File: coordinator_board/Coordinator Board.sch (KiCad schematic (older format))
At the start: 9 parts, among them P1 LCD, P2 Serial

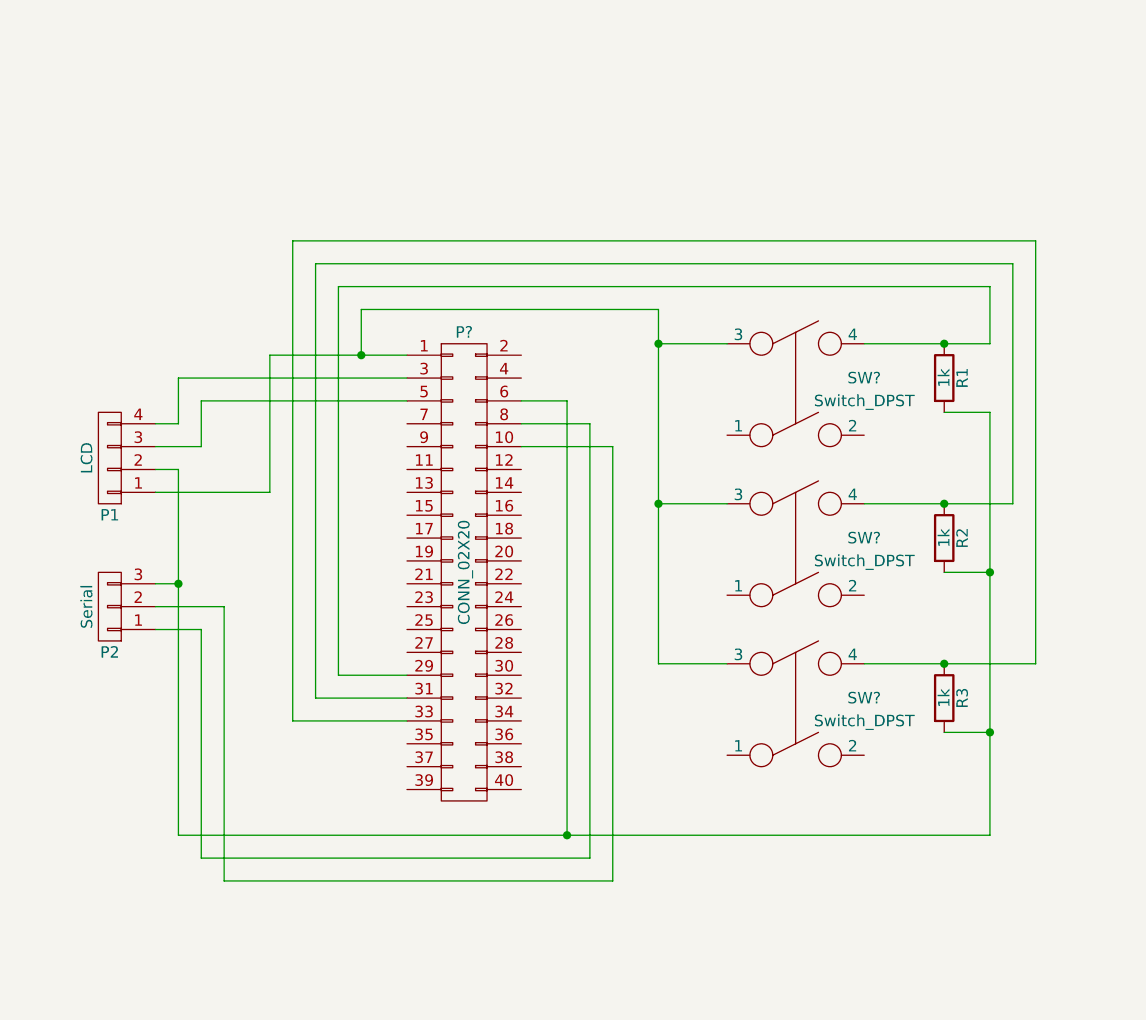
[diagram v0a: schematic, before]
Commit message: Finished v1 of the board
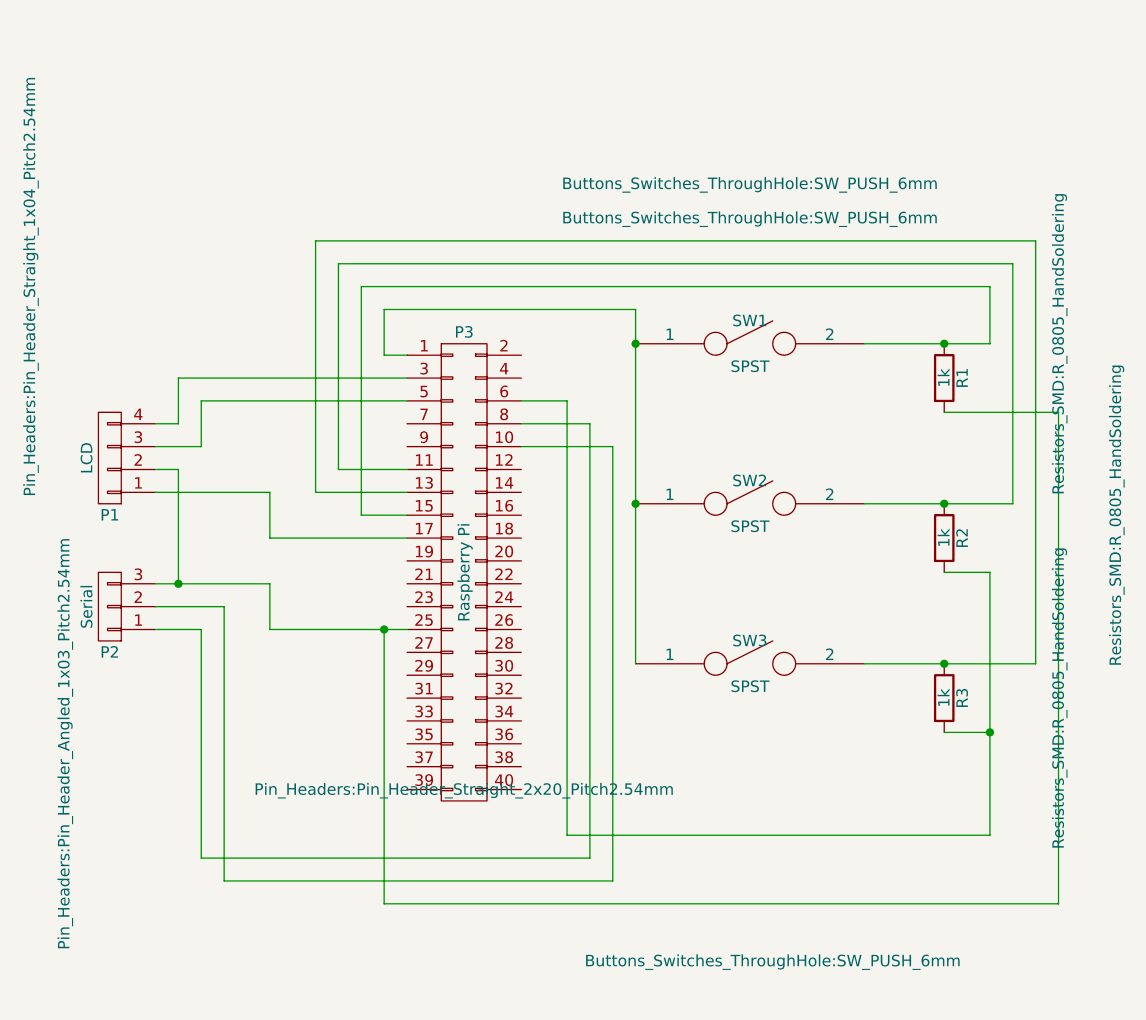
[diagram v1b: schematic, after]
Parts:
- removed SW? (x3): Switch_DPST, symbol Switch_DPST
- added SW1, SW2, SW3: SPST, Buttons_Switches_ThroughHole:SW_PUSH_6mm, symbol SPST
- P1: footprint (none) -> Pin_Headers:Pin_Header_Straight_1x04_Pitch2.54mm
- P2: footprint (none) -> Pin_Headers:Pin_Header_Angled_1x03_Pitch2.54mm
- P3: renamed from P?; value CONN_02X20 -> Raspberry Pi; footprint (none) -> Pin_Headers:Pin_Header_Straight_2x20_Pitch2.54mm
- R1, R2, R3: footprint (none) -> Resistors_SMD:R_0805_HandSoldering
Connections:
- net at P3.1 (P1): now also SW1.1, SW2.1, SW3.1; no longer P1.1 (P1)
- net at P3.11 (P11): now also R2.1, SW2.2
- net at P3.13 (P13): now also R3.1, SW3.2
- net at P3.15 (P15): now also R1.1, SW1.2
- net at P3.17 (P17): now also P1.1 (P1)
- net at P3.25 (P25): now also P1.2 (P2), P2.3 (P3), R1.2
- net at P3.29 (P29): no longer R1.1
- net at P3.31 (P31): no longer R2.1
- net at P3.33 (P33): no longer R3.1
- net at P3.6 (P6), R2.2, R3.2: no longer P1.2 (P2), P2.3 (P3), R1.2
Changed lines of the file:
@@
 $EndDescr
 $Comp
-L CONN_02X20 P?
+L CONN_02X20 P3
 U 1 1 586759B9
 P 3950 3850
-F 0 "P?" H 3950 4900 50  0000 C CNN
-F 1 "CONN_02X20" V 3950 3850 50  0000 C CNN
-F 2 "" H 3950 2900 50  0000 C CNN
+F 0 "P3" H 3950 4900 50  0000 C CNN
+F 1 "Raspberry Pi" V 3950 3850 50  0000 C CNN
+F 2 "Pin_Headers:Pin_Header_Straight_2x20_Pitch2.54mm" H 3950 2900 50  0000 C CNN
 F 3 "" H 3950 2900 50  0000 C CNN
 	1    3950 3850
 	1    0    0    -1
 $EndComp
-$Comp
-L Switch_DPST SW?
-U 1 1 58675A3B
-P 5400 3050
-F 0 "SW?" H 5700 3100 50  0000 C CNN
-F 1 "Switch_DPST" H 5700 3000 50  0000 C CNN
-F 2 "" H 5400 3050 50  0000 C CNN
-F 3 "" H 5400 3050 50  0000 C CNN
-	1    5400 3050
-	1    0    0    -1
-$EndComp
-$Comp
-L Switch_DPST SW?
-U 1 1 58675A65
-P 5400 3750
-F 0 "SW?" H 5700 3800 50  0000 C CNN
-F 1 "Switch_DPST" H 5700 3700 50  0000 C CNN
-F 2 "" H 5400 3750 50  0000 C CNN
-F 3 "" H 5400 3750 50  0000 C CNN
-	1    5400 3750
-	1    0    0    -1
-$EndComp
-$Comp
-L Switch_DPST SW?
-U 1 1 58675A90
-P 5400 4450
-F 0 "SW?" H 5700 4500 50  0000 C CNN
-F 1 "Switch_DPST" H 5700 4400 50  0000 C CNN
-F 2 "" H 5400 4450 50  0000 C CNN
-F 3 "" H 5400 4450 50  0000 C CNN
-	1    5400 4450
-	1    0    0    -1
-$EndComp
-Wire Wire Line
-	3100 2900 3700 2900
-Wire Wire Line
-	3500 2900 3500 2700
-Wire Wire Line
-	3500 2700 4800 2700
-Wire Wire Line
-	4800 2700 4800 4250
-Wire Wire Line
-	4800 4250 5100 4250
-Wire Wire Line
-	5100 2850 4800 2850
-Connection ~ 4800 2850
-Wire Wire Line
-	5100 3550 4800 3550
-Connection ~ 4800 3550
+Wire Wire Line
+	3600 2900 3700 2900
+Wire Wire Line
+	3600 2700 3600 2900
+Wire Wire Line
+	3100 3500 3100 3700
 Wire Wire Line
 	4200 3100 4400 3100
 Wire Wire Line
 	4400 3100 4400 5000
-Wire Wire Line
-	2700 5000 6250 5000
 $Comp
 L R R1
@@
 F 0 "R1" V 6130 3000 50  0000 C CNN
 F 1 "1k" V 6050 3000 50  0000 C CNN
-F 2 "" V 5980 3000 50  0000 C CNN
+F 2 "Resistors_SMD:R_0805_HandSoldering" V 6550 3150 50  0000 C CNN
 F 3 "" H 6050 3000 50  0000 C CNN
 	1    6050 3000
@@
 F 0 "R2" V 6130 3700 50  0000 C CNN
 F 1 "1k" V 6050 3700 50  0000 C CNN
-F 2 "" V 5980 3700 50  0000 C CNN
+F 2 "Resistors_SMD:R_0805_HandSoldering" V 6800 3800 50  0000 C CNN
 F 3 "" H 6050 3700 50  0000 C CNN
 	1    6050 3700
@@
 F 0 "R3" V 6130 4400 50  0000 C CNN
 F 1 "1k" V 6050 4400 50  0000 C CNN
-F 2 "" V 5980 4400 50  0000 C CNN
+F 2 "Resistors_SMD:R_0805_HandSoldering" V 6550 4400 50  0000 C CNN
 F 3 "" H 6050 4400 50  0000 C CNN
 	1    6050 4400
@@
 	5700 4250 6450 4250
 Wire Wire Line
-	6250 3150 6050 3150
-Wire Wire Line
-	6050 4550 6250 4550
+	6250 4550 6050 4550
 Connection ~ 6250 4550
 Wire Wire Line
-	6250 5000 6250 3150
-Wire Wire Line
 	6250 3850 6050 3850
-Connection ~ 6250 3850
-Wire Wire Line
-	3700 4300 3400 4300
-Wire Wire Line
-	3400 4300 3400 2600
-Wire Wire Line
-	3400 2600 6250 2600
-Wire Wire Line
-	3700 4400 3300 4400
-Wire Wire Line
-	3300 4400 3300 2500
-Wire Wire Line
-	3300 2500 6350 2500
-Wire Wire Line
-	6350 2500 6350 3550
-Connection ~ 6050 3550
-Wire Wire Line
-	3700 4500 3200 4500
-Wire Wire Line
-	3200 4500 3200 2400
-Wire Wire Line
-	3200 2400 6450 2400
-Wire Wire Line
-	6450 2400 6450 4250
-Connection ~ 6050 4250
-Wire Wire Line
-	6250 2600 6250 2850
-Connection ~ 6050 2850
 $Comp
 L CONN_01X04 P1
@@
 F 0 "P1" H 2400 3600 50  0000 C CNN
 F 1 "LCD" V 2500 3350 50  0000 C CNN
-F 2 "" H 2400 3350 50  0000 C CNN
+F 2 "Pin_Headers:Pin_Header_Straight_1x04_Pitch2.54mm" V 2750 2600 50  0000 C CNN
 F 3 "" H 2400 3350 50  0000 C CNN
 	1    2400 3350
@@
 $EndComp
 Wire Wire Line
-	3100 2900 3100 3500
-Wire Wire Line
 	3100 3500 2600 3500
-Connection ~ 3500 2900
-Wire Wire Line
-	2700 5000 2700 3400
+Wire Wire Line
+	2700 3400 2700 3900
 Wire Wire Line
 	2700 3400 2600 3400
-Connection ~ 4400 5000
 Wire Wire Line
 	3700 3100 2800 3100
@@
 F 0 "P2" H 2400 4200 50  0000 C CNN
 F 1 "Serial" V 2500 4000 50  0000 C CNN
-F 2 "" H 2400 4000 50  0000 C CNN
+F 2 "Pin_Headers:Pin_Header_Angled_1x03_Pitch2.54mm" V 2600 4600 50  0000 C CNN
 F 3 "" H 2400 4000 50  0000 C CNN
 	1    2400 4000
@@
 	2900 4000 2600 4000
 Wire Wire Line
-	2600 3900 2700 3900
+	2600 3900 3100 3900
 Connection ~ 2700 3900
+Wire Wire Line
+	3500 2600 3500 3600
+Wire Wire Line
+	3500 2600 6250 2600
+Wire Wire Line
+	6250 2600 6250 2850
+Connection ~ 6050 2850
+Wire Wire Line
+	3700 3400 3400 3400
+Wire Wire Line
+	3400 3400 3400 2500
+Wire Wire Line
+	3400 2500 6350 2500
+Wire Wire Line
+	6350 2500 6350 3550
+Connection ~ 6050 3550
+Wire Wire Line
+	3700 3500 3300 3500
+Wire Wire Line
+	3300 3500 3300 2400
+Wire Wire Line
+	3300 2400 6450 2400
+Wire Wire Line
+	6450 2400 6450 4250
+Connection ~ 6050 4250
+$Comp
+L SPST SW1
+U 1 1 587594B8
+P 5200 2850
+F 0 "SW1" H 5200 2950 50  0000 C CNN
+F 1 "SPST" H 5200 2750 50  0000 C CNN
+F 2 "Buttons_Switches_ThroughHole:SW_PUSH_6mm" H 5200 3550 50  0000 C CNN
+F 3 "" H 5200 2850 50  0000 C CNN
+	1    5200 2850
+	1    0    0    -1
+$EndComp
+$Comp
+L SPST SW2
+U 1 1 587595F9
+P 5200 3550
+F 0 "SW2" H 5200 3650 50  0000 C CNN
+F 1 "SPST" H 5200 3450 50  0000 C CNN
+F 2 "Buttons_Switches_ThroughHole:SW_PUSH_6mm" H 5200 4800 50  0000 C CNN
+F 3 "" H 5200 3550 50  0000 C CNN
+	1    5200 3550
+	1    0    0    -1
+$EndComp
+$Comp
+L SPST SW3
+U 1 1 58759632
+P 5200 4250
+F 0 "SW3" H 5200 4350 50  0000 C CNN
+F 1 "SPST" H 5200 4150 50  0000 C CNN
+F 2 "Buttons_Switches_ThroughHole:SW_PUSH_6mm" H 5300 2950 50  0000 C CNN
+F 3 "" H 5200 4250 50  0000 C CNN
+	1    5200 4250
+	1    0    0    -1
+$EndComp
+Wire Wire Line
+	3600 2700 4700 2700
+Wire Wire Line
+	4700 2700 4700 4250
+Connection ~ 4700 2850
+Connection ~ 4700 3550
+Wire Wire Line
+	3500 3600 3700 3600
+Wire Wire Line
+	3100 3700 3700 3700
+Wire Wire Line
+	6050 3150 6550 3150
+Wire Wire Line
+	6550 3150 6550 5300
+Wire Wire Line
+	6550 5300 3600 5300
+Wire Wire Line
+	3600 5300 3600 4100
+Wire Wire Line
+	3100 4100 3700 4100
+Wire Wire Line
+	6250 3850 6250 5000
+Wire Wire Line
+	6250 5000 4400 5000
+Wire Wire Line
+	3100 3900 3100 4100
+Connection ~ 3600 4100
 $EndSCHEMATC
